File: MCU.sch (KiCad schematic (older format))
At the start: 13 parts, among them J1 Conn_01x05, J2 Conn_01x14, U2 STM32F072RBTx

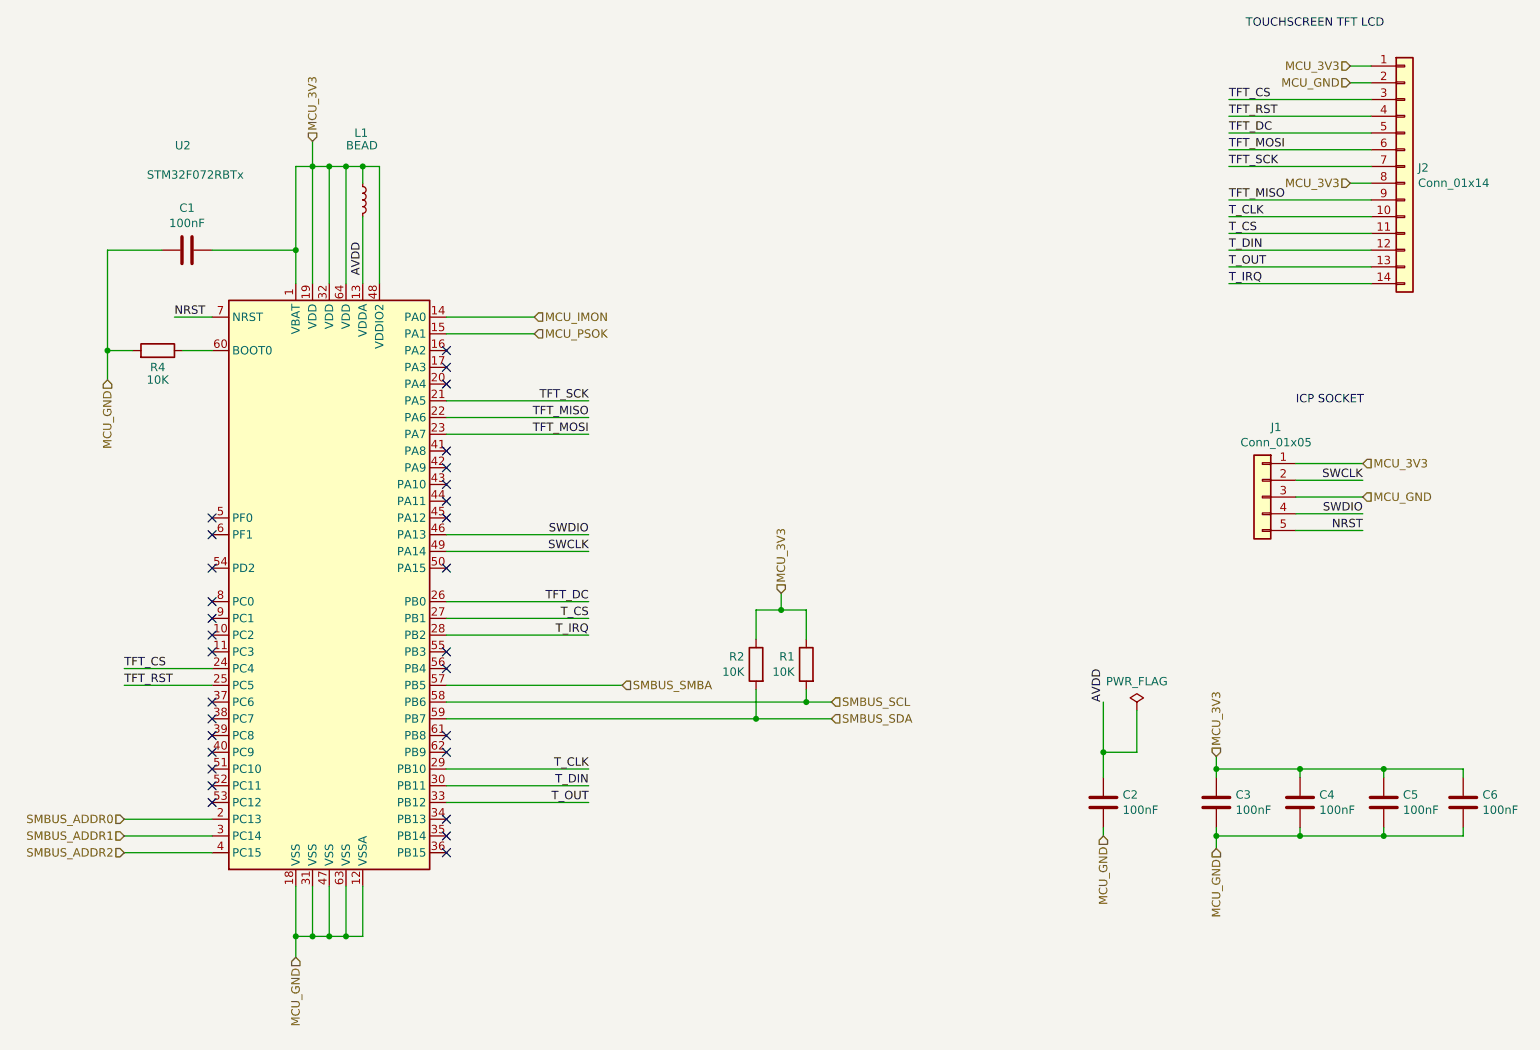
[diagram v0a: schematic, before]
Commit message: layout draft
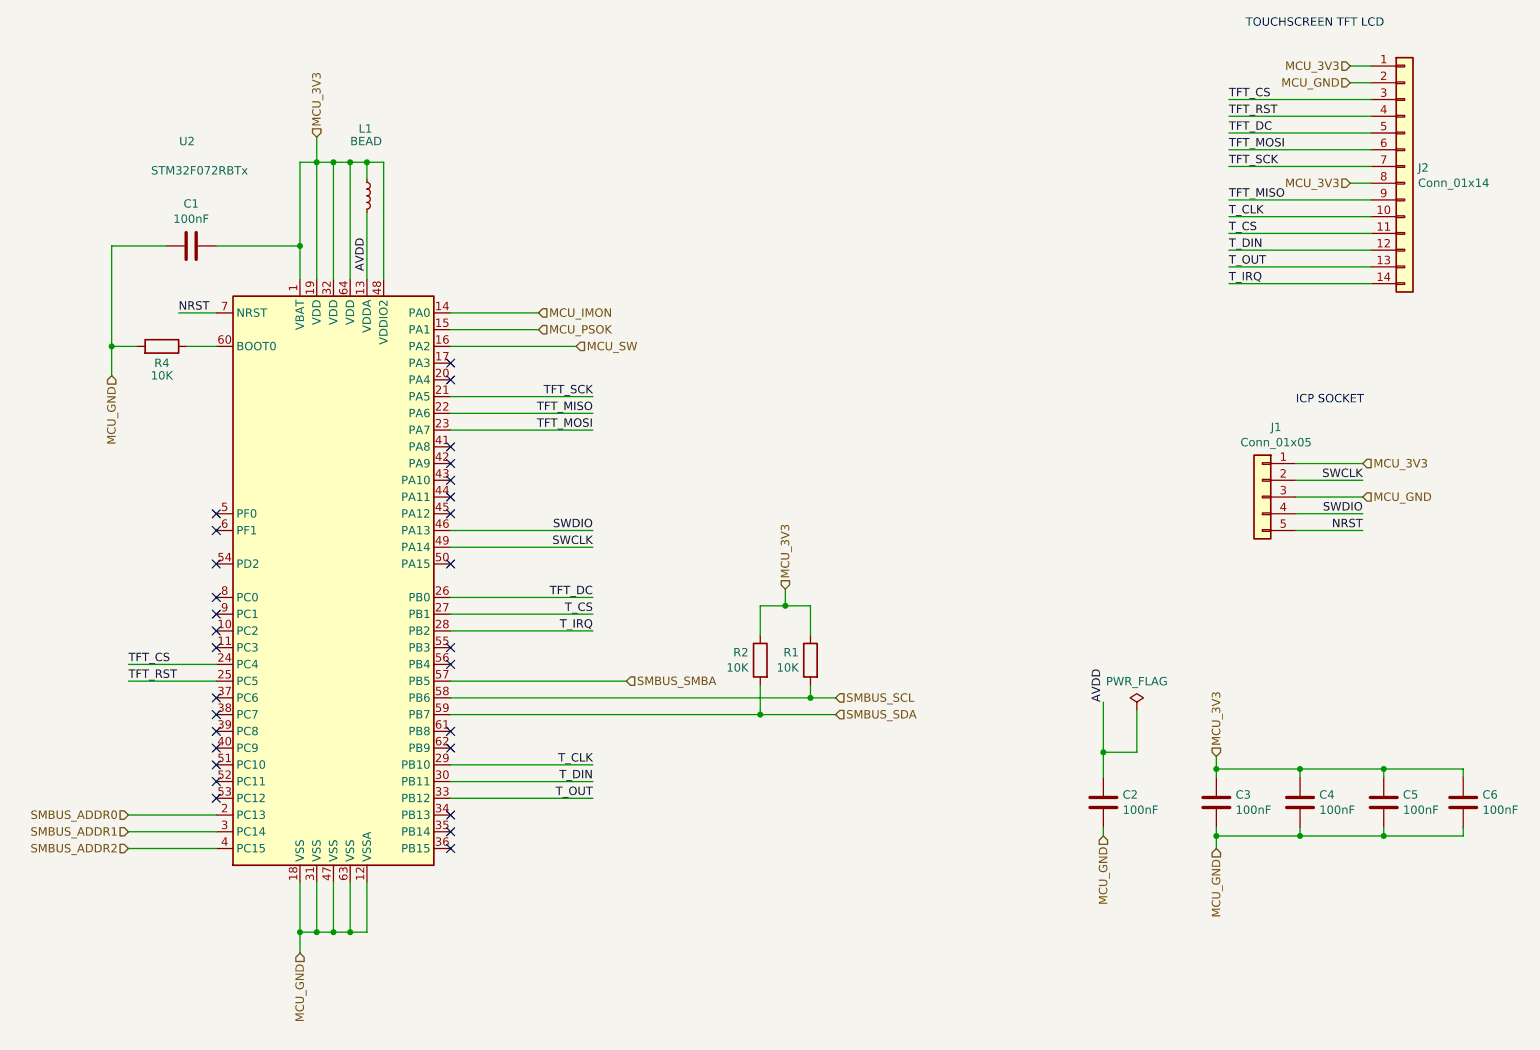
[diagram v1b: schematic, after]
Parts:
- J1: footprint (none) -> Connector_PinHeader_2.54mm:PinHeader_1x05_P2.54mm_Vertical
- J2: footprint (none) -> Connector_PinHeader_2.54mm:PinHeader_1x14_P2.54mm_Vertical
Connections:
- net MCU_SW: now reaches U2.16 (PA2)
- no-connect marks 30 -> 29
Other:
- moved on the sheet: C1, L1, R1, R2, R4, U2
